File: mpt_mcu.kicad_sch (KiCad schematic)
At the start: 11 parts, among them SW2 KMR421GULCLFS, SW3 KMR421GULCLFS, U4 ESP32-S3-WROOM-1-N4R2

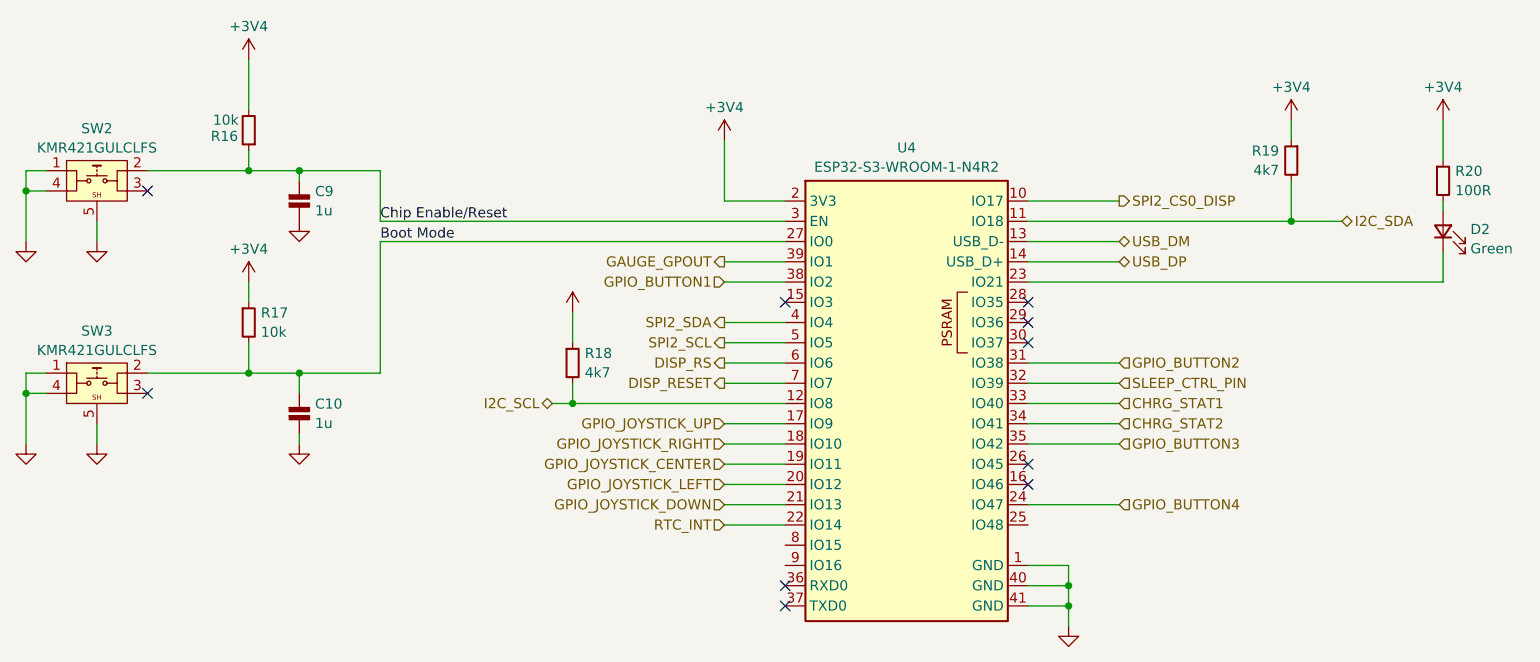
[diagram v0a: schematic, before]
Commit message: Started routing of componentes
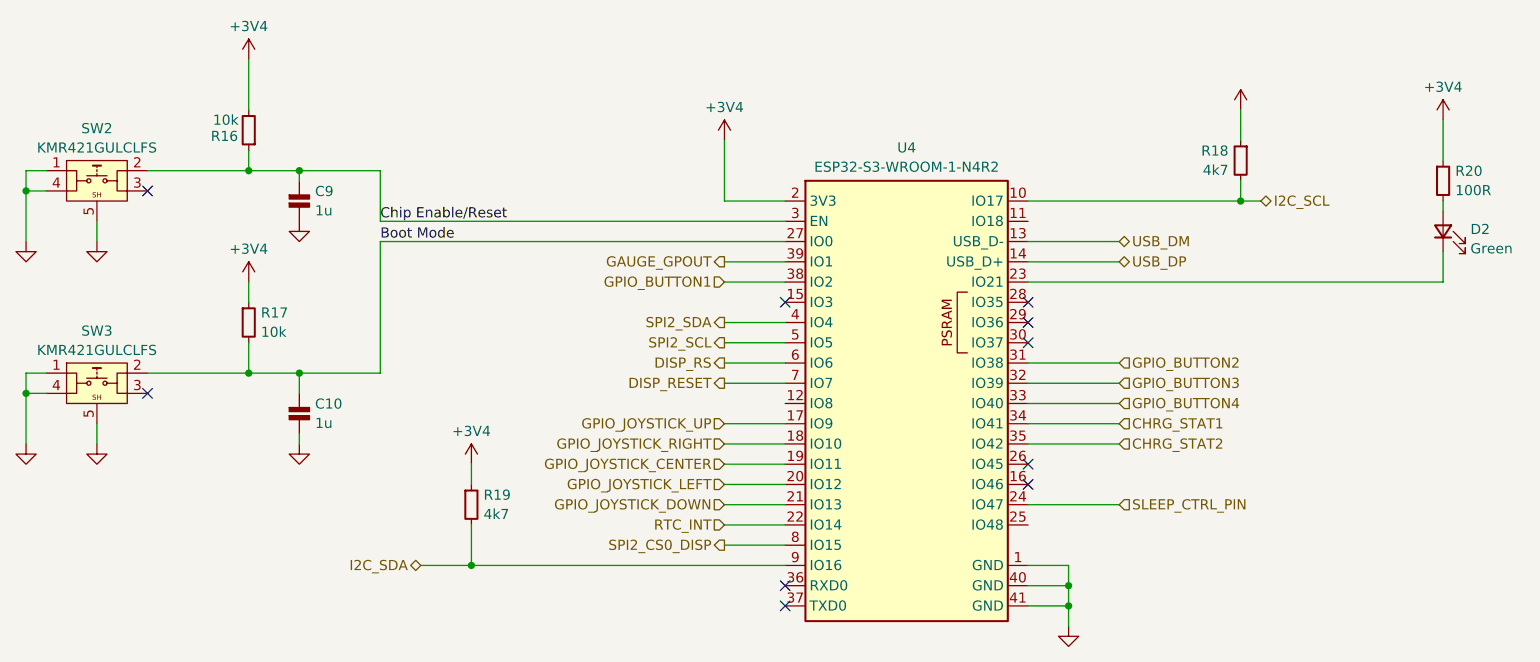
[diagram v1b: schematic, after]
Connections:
- net CHRG_STAT1: now also U4.34 (IO41); no longer U4.33 (IO40)
- net CHRG_STAT2: now also U4.35 (IO42); no longer U4.34 (IO41)
- net GPIO_BUTTON3: now also U4.32 (IO39); no longer U4.35 (IO42)
- net GPIO_BUTTON4: now also U4.33 (IO40); no longer U4.24 (IO47)
- net I2C_SCL: now also U4.10 (IO17); no longer U4.12 (IO8)
- net I2C_SDA: now also U4.9 (IO16); no longer U4.11 (IO18)
- net SLEEP_CTRL_PIN: now also U4.24 (IO47); no longer U4.32 (IO39)
- net SPI2_CS0_DISP: now also U4.8 (IO15); no longer U4.10 (IO17)
